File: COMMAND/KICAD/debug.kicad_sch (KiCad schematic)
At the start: 1 part, among them J2 FTSH-107-01-X-DV

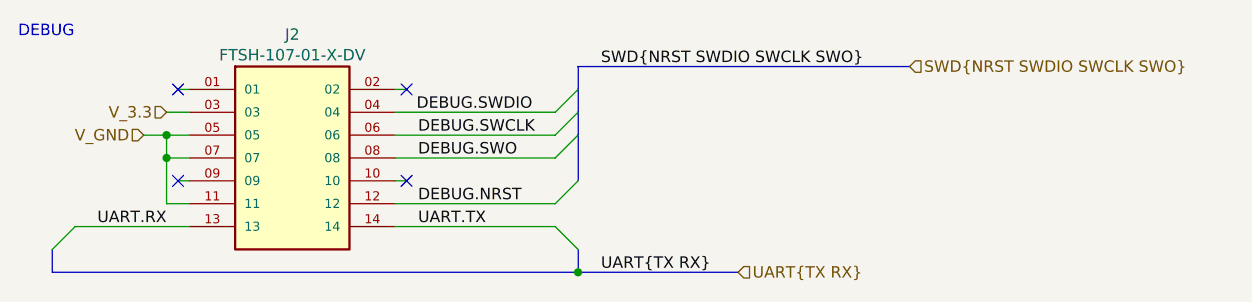
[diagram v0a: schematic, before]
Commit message: schematic design
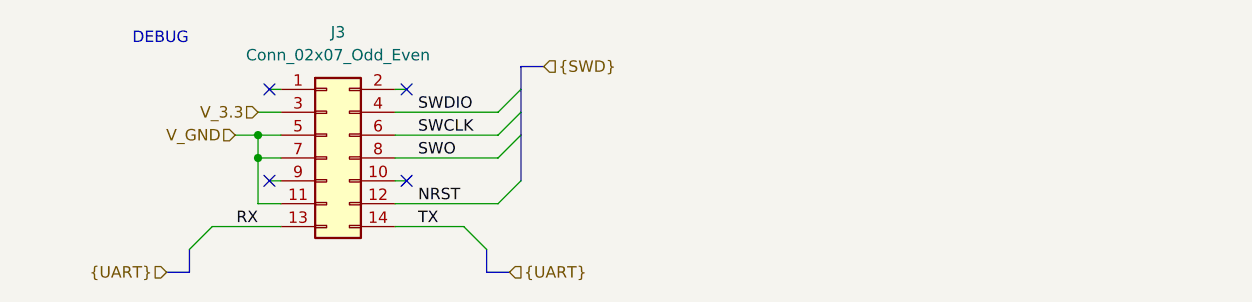
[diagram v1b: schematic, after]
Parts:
- removed J2: FTSH-107-01-X-DV, symbol CUBESAT:FTSH-107-XX-X-DV
- added J3: Conn_02x07_Odd_Even, symbol Connector_Generic:Conn_02x07_Odd_Even
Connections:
- net V_3.3: now also J3.3 (Pin_3)
- net V_GND: now also J3.11 (Pin_11), J3.5 (Pin_5), J3.7 (Pin_7)
- new net NRST: J3.12 (Pin_12)
- new net RX: J3.13 (Pin_13)
- new net SWCLK: J3.6 (Pin_6)
- new net SWDIO: J3.4 (Pin_4)
- new net SWO: J3.8 (Pin_8)
- new net TX: J3.14 (Pin_14)
